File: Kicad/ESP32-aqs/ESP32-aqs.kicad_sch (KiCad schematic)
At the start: 23 parts, among them J1 UART Connector, J2 Conn SEN55, SW1 RESET, SW2 BOOT, U1 LD1117S33TR_SOT223, U2 ESP32-WROOM-32, U3 SGP41-D-R4, U4 SX1276S8S+T-X1

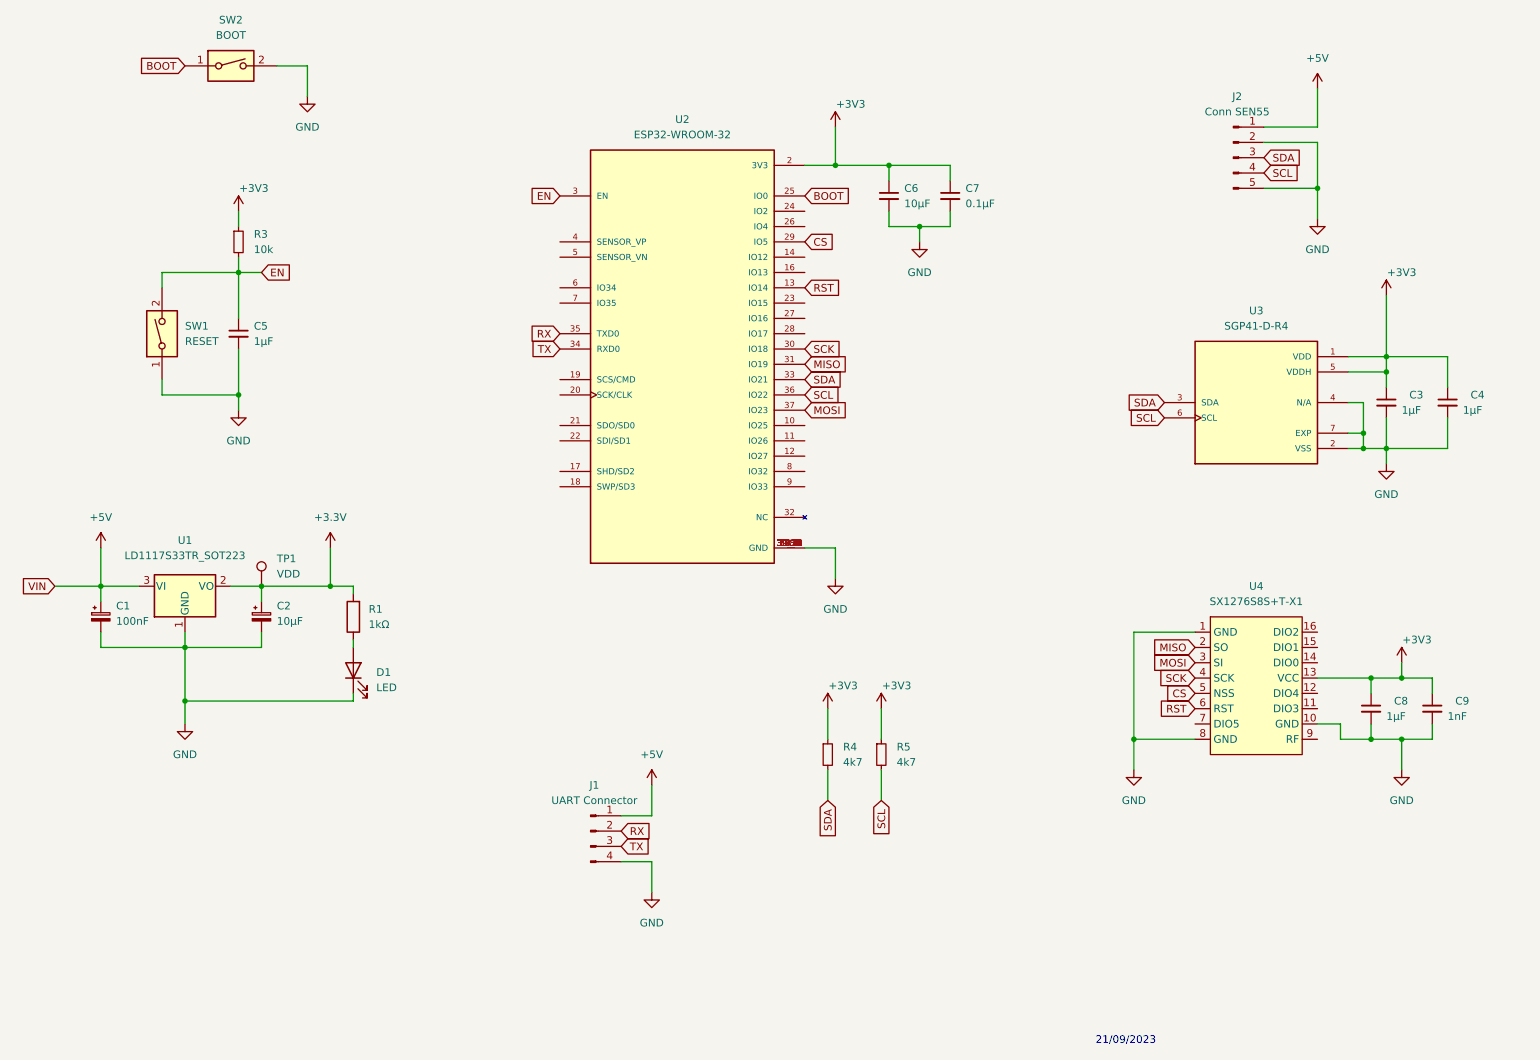
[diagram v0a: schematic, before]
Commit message: Add files via upload
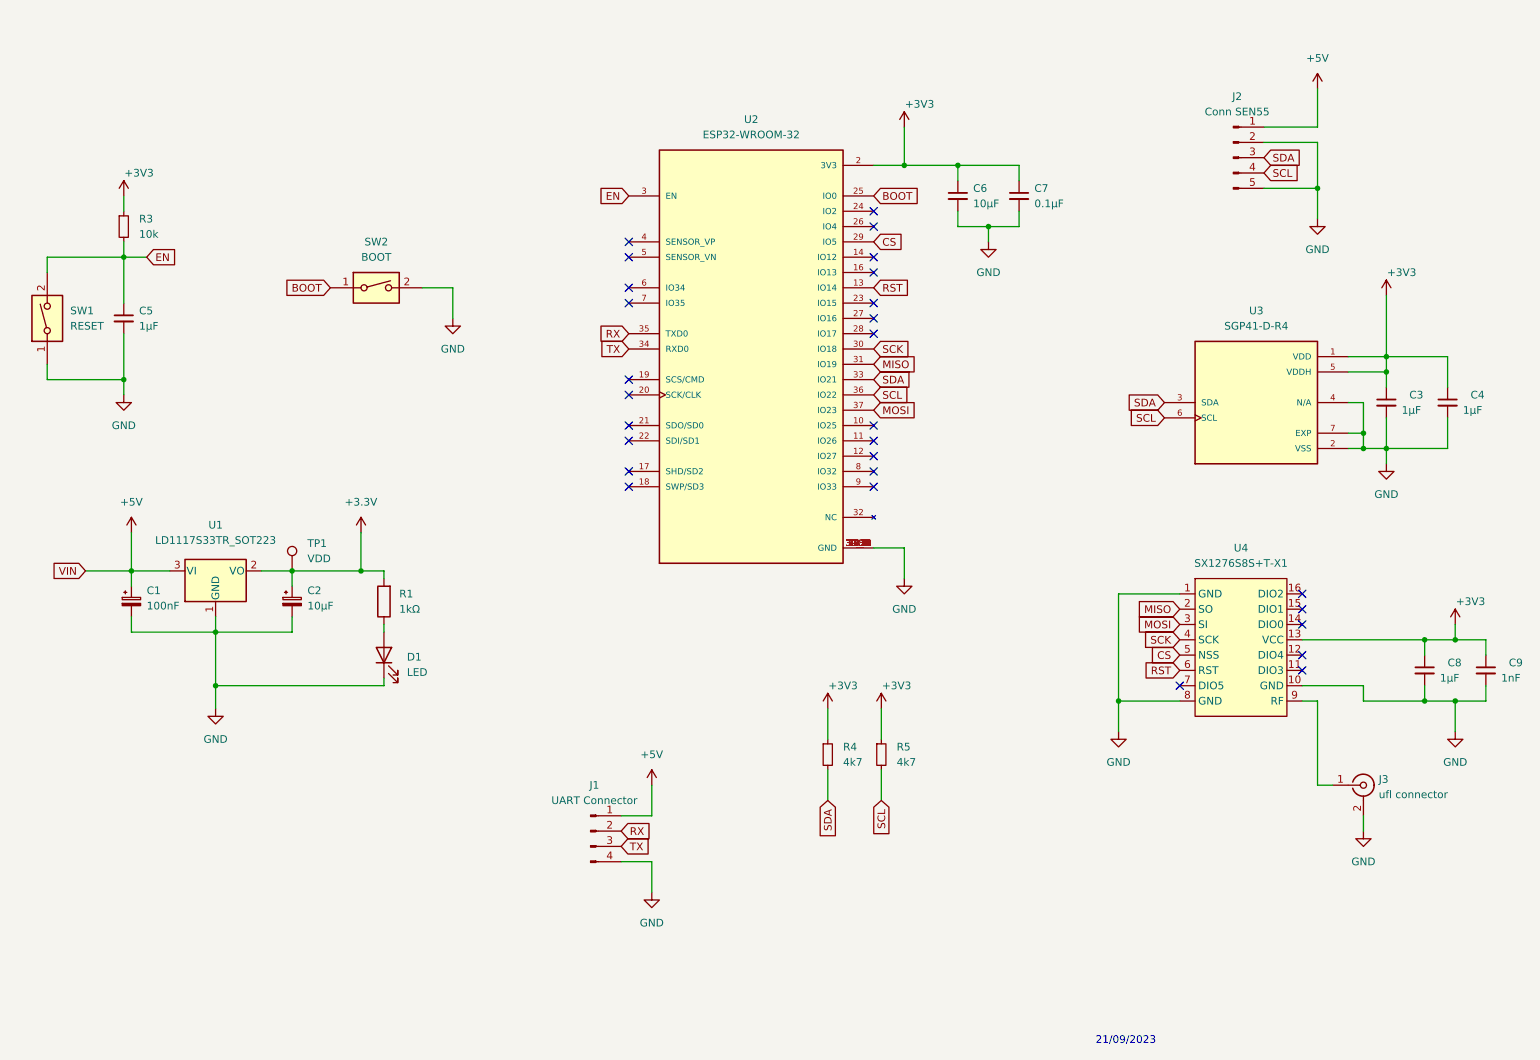
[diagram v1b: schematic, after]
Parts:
- added J3: ufl connector, Connector_Coaxial:U.FL_Molex_MCRF_73412-0110_Vertical, symbol Connector:Conn_Coaxial
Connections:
- net GND: now also J3.2 (Ext)
- net at U4.9 (RF): now also J3.1 (In)
- no-connect marks 0 -> 28
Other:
- moved on the sheet: C1, C2, C5, C6, C7, C8, C9, D1, R1, R3, SW1, SW2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
